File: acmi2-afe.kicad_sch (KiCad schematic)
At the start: 14 parts

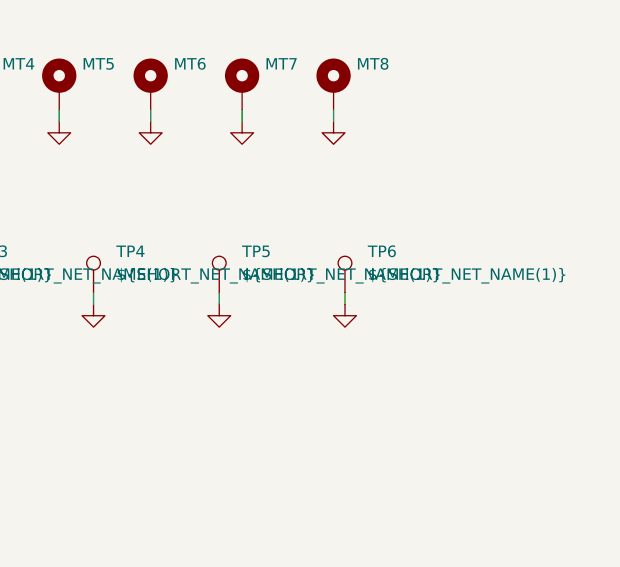
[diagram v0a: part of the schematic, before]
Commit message: Finish routing
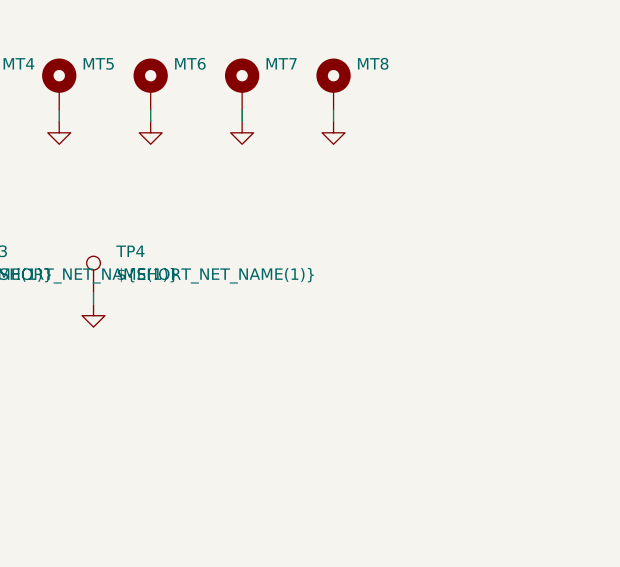
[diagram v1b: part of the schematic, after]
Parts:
- removed TP5, TP6: ${SHORT_NET_NAME(1)}, My Footprints:TestPoint_RCS-0C, symbol Connector:TestPoint
